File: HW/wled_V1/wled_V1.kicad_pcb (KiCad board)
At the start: 2 copper layers, 52 x 78 mm, 25 parts, among them IC1 SN74AHCT125DR, J1 694106301002

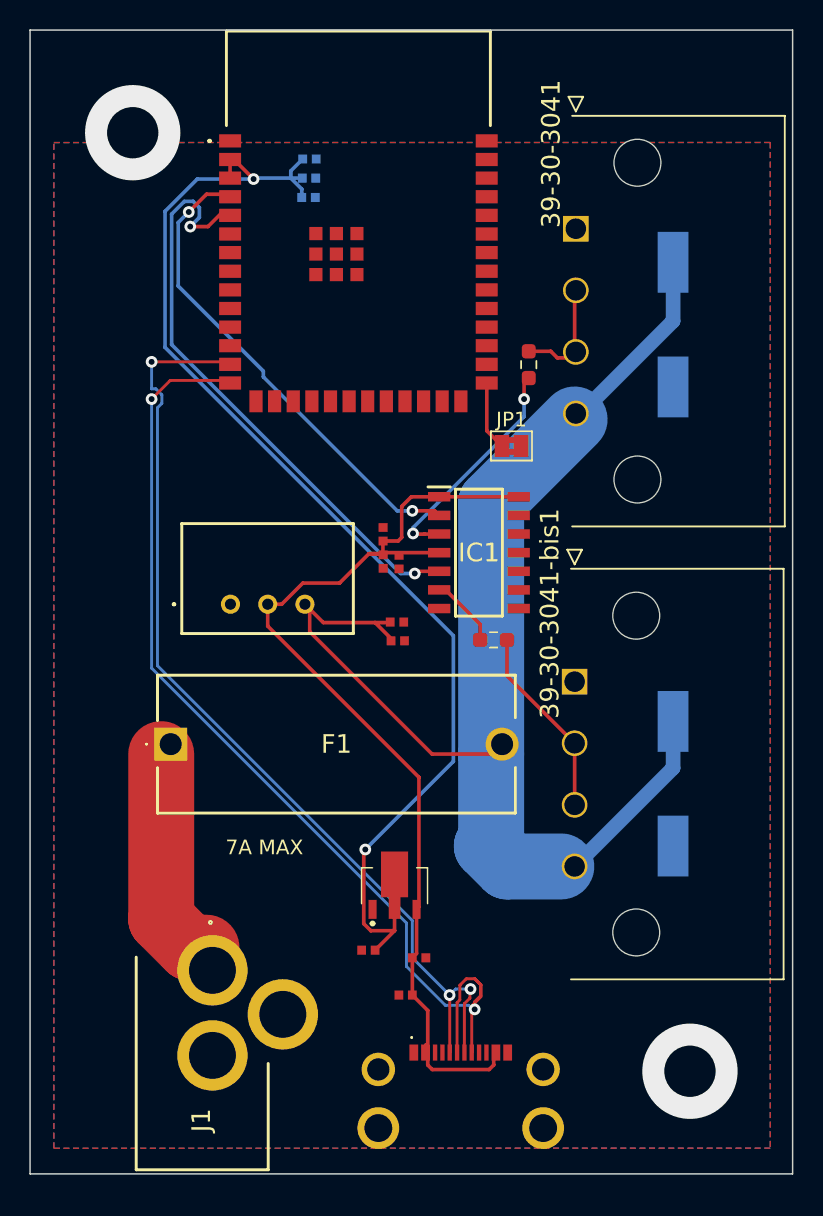
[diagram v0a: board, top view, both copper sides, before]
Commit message: route
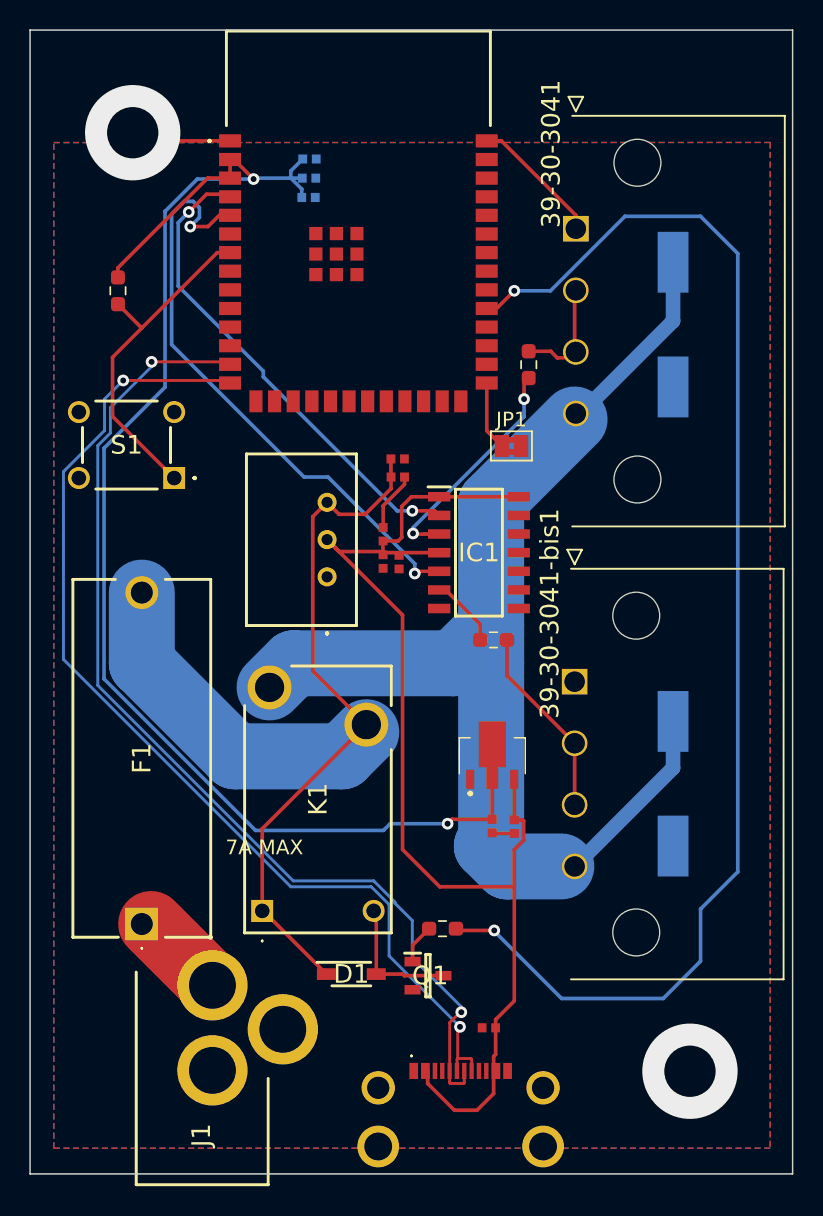
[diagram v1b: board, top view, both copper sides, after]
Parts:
- added D1: 1N4148W_R1_00001, SamacSys_Parts:SOD3816X135N, F.Cu at (21.9, 64.4)
- added K1: AHQSH112LM1F00G, SamacSys_Parts:AHQSH112LM1F00G, F.Cu at (15.8, 60.1)
- added Q1: MMBT3904-7-F, SamacSys_Parts:SOT96P240X110-3N, F.Cu at (27.1, 64.5)
- added RN73H1JTTD1002F1: 10k, Resistor_SMD:R_0603_1608Metric_Pad0.98x0.95mm_HandSolder, F.Cu at (5.99, 17.8)
- added RN73H1JTTD1002F50: 10k, Resistor_SMD:R_0603_1608Metric_Pad0.98x0.95mm_HandSolder, F.Cu at (28.1, 61.3)
- added S1: TS14-1212-140-BK-160-SCR-D, SamacSys_Parts:TS0266160BK260LCRD, F.Cu at (9.83, 30.5)
- moved F1 12.4 mm to (7.62, 61.0), turned to 90 degrees
- moved C15 12.0 mm to (31.5, 54.3), turned to -90 degrees
- moved C13 11.2 mm to (25.1, 30.5)
- moved C3 11.1 mm to (25.1, 29.2)
- moved AZ1117CR-3.3TRG1 11.1 mm to (31.5, 48.3)
- moved C11 11.1 mm to (33.0, 54.3), turned to -90 degrees
- moved TSR-1-2450 6.85 mm to (20.3, 37.3), turned to 90 degrees
- moved C9 6.10 mm to (31.3, 68.0)
- moved 216990-0002 1.26 mm to (29.4, 73.8)
- moved J1 1.02 mm to (16.2, 78.7)
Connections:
- 39-30-3041 pad 4: +12V -> 12v_commuted
- 39-30-3041-bis1 pad 4: +12V -> 12v_commuted
- C5 pad 1: +12V -> 12v_commuted
- C8 pad 2: +12V -> 12v_commuted
- ESP32-S3-WROOM-1-N8 pad 31: unconnected-(ESP32-S3-WROOM-1-N8-GPIO38/FSPIWP/SUBSPIWP-Pad31) -> D6
- ESP32-S3-WROOM-1-N8 pad 7: D6 -> GPIO7
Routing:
- net D6: track 0.00 -> 89.9 mm, vias 0 -> 2
- net 12v_commuted: track 0.00 -> 80.2 mm
- net GPIO7: track 0.00 -> 23.2 mm
- net GND: track 1.40 -> 22.9 mm
- net +12V: track 88.2 -> 69.8 mm
- net +3.3V: track 82.0 -> 95.3 mm
- net +5V: track 69.0 -> 81.9 mm
- net Net-(D1-A): track 0.00 -> 9.00 mm
- net Net-(J1-POWER): track 15.1 -> 6.55 mm
- net D-: track 67.4 -> 71.7 mm, vias 3 -> 2
- net Net-(Q1-B): track 0.00 -> 2.71 mm
- net D+: track 71.4 -> 72.4 mm
